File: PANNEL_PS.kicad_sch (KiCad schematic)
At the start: 19 parts, among them IC30 TPS25940ARVCR, IC31 INA226AIDGSR

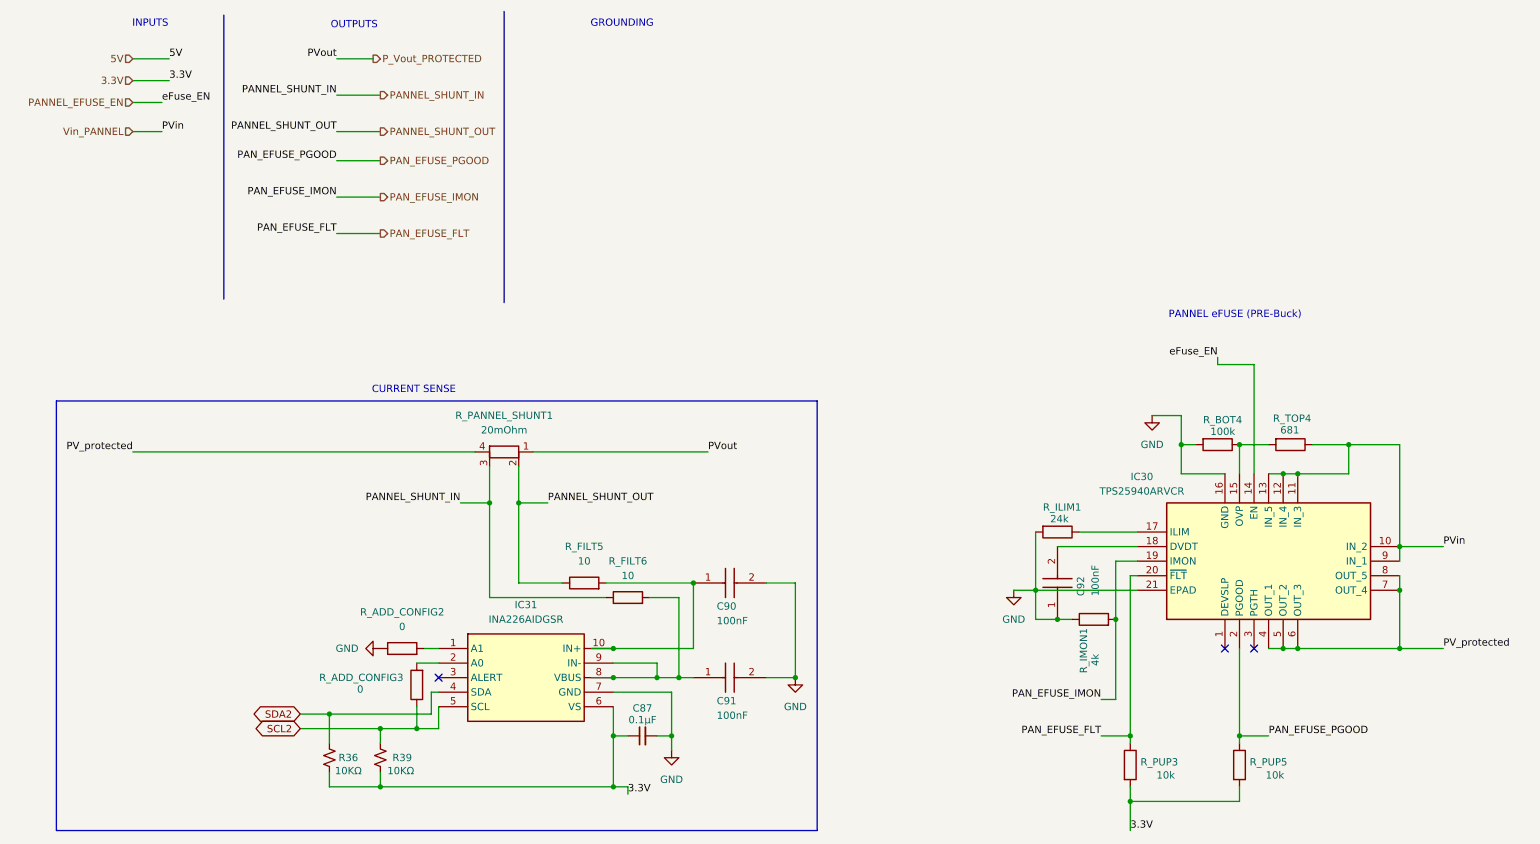
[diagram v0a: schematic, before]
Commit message: Big final PCU PCB design
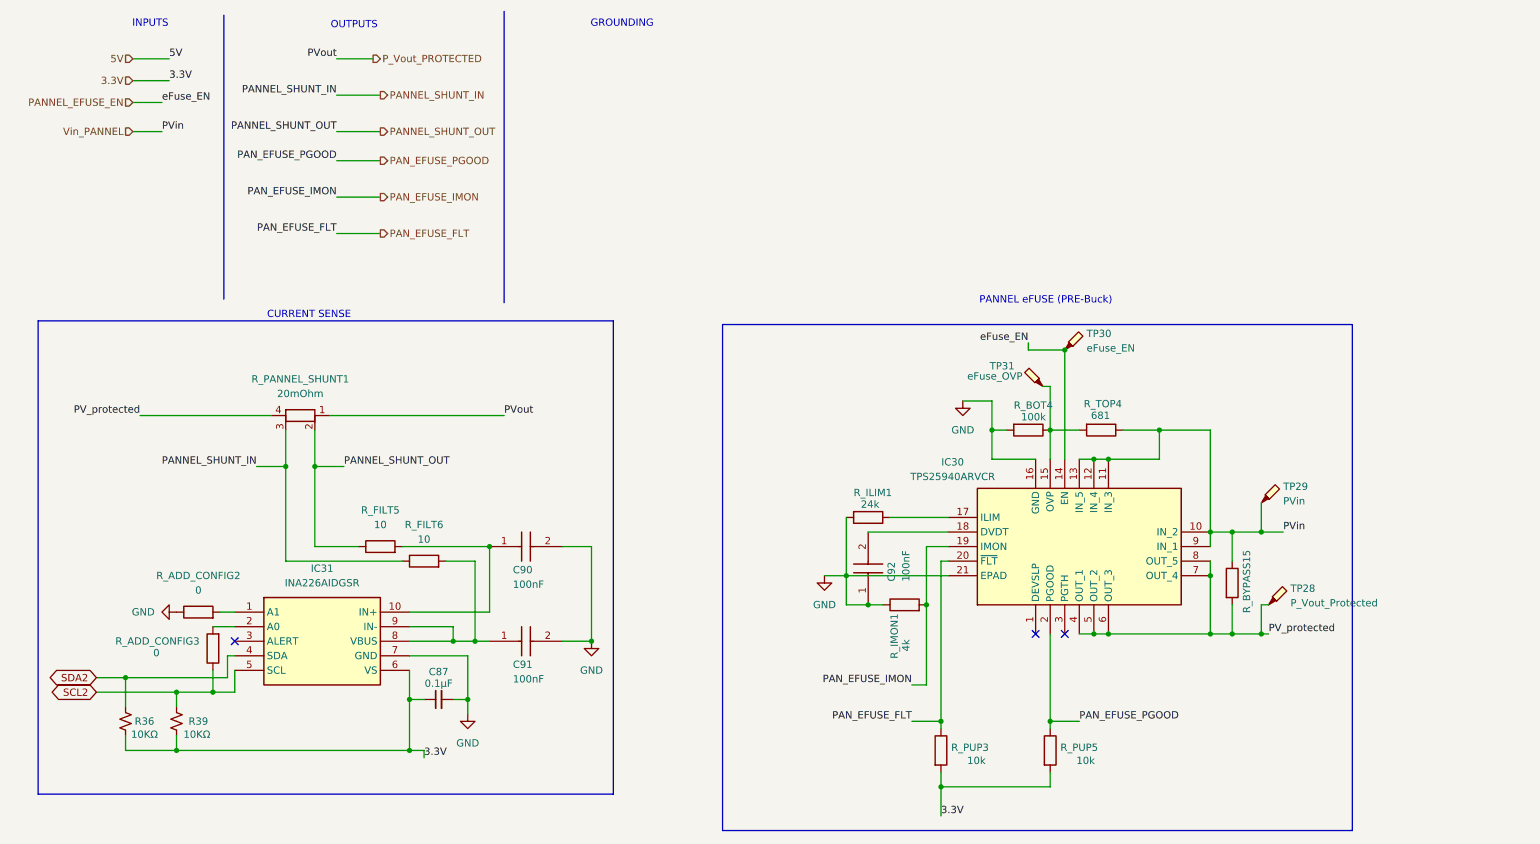
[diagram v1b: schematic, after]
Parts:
- added R_BYPASS15: 0, Resistor_SMD:R_0603_1608Metric, symbol Device:R
- added TP28: P_Vout_Protected, TestPoint:TestPoint_Pad_D2.0mm, symbol Connector:TestPoint_Probe
- added TP29: PVin, TestPoint:TestPoint_Pad_D2.0mm, symbol Connector:TestPoint_Probe
- added TP30: eFuse_EN, TestPoint:TestPoint_Pad_D2.0mm, symbol Connector:TestPoint_Probe
- added TP31: eFuse_OVP, TestPoint:TestPoint_Pad_D2.0mm, symbol Connector:TestPoint_Probe
- C90, C91, C92: footprint C0603_Commercial -> Capacitor_SMD:C_0603_1608Metric
- R_PANNEL_SHUNT1: footprint (none) -> Resistor_SMD:R_Shunt_Vishay_WSKW0612
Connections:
- net PANNEL_EFUSE_EN: now also TP30.1
- net PV_protected: now also R_BYPASS15.2, TP28.1
- net Vin_PANNEL: now also R_BYPASS15.1, TP29.1
- net at IC30.15 (OVP), R_BOT4.1, R_TOP4.2: now also TP31.1
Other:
- moved on the sheet: C87, C90, C91, C92, IC30, IC31, R36, R39, R_ADD_CONFIG2, R_ADD_CONFIG3, R_BOT4, R_FILT5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
